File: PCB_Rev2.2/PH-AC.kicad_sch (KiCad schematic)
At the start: 42 parts, among them J1 USB_C_Receptacle_USB2.0_16P, J2 Conn_01x03, SW1 SW_Push, U1 RP2040, U2 AMS1117-3.3, U3 W25Q16JVSS, Y1 Crystal_GND24

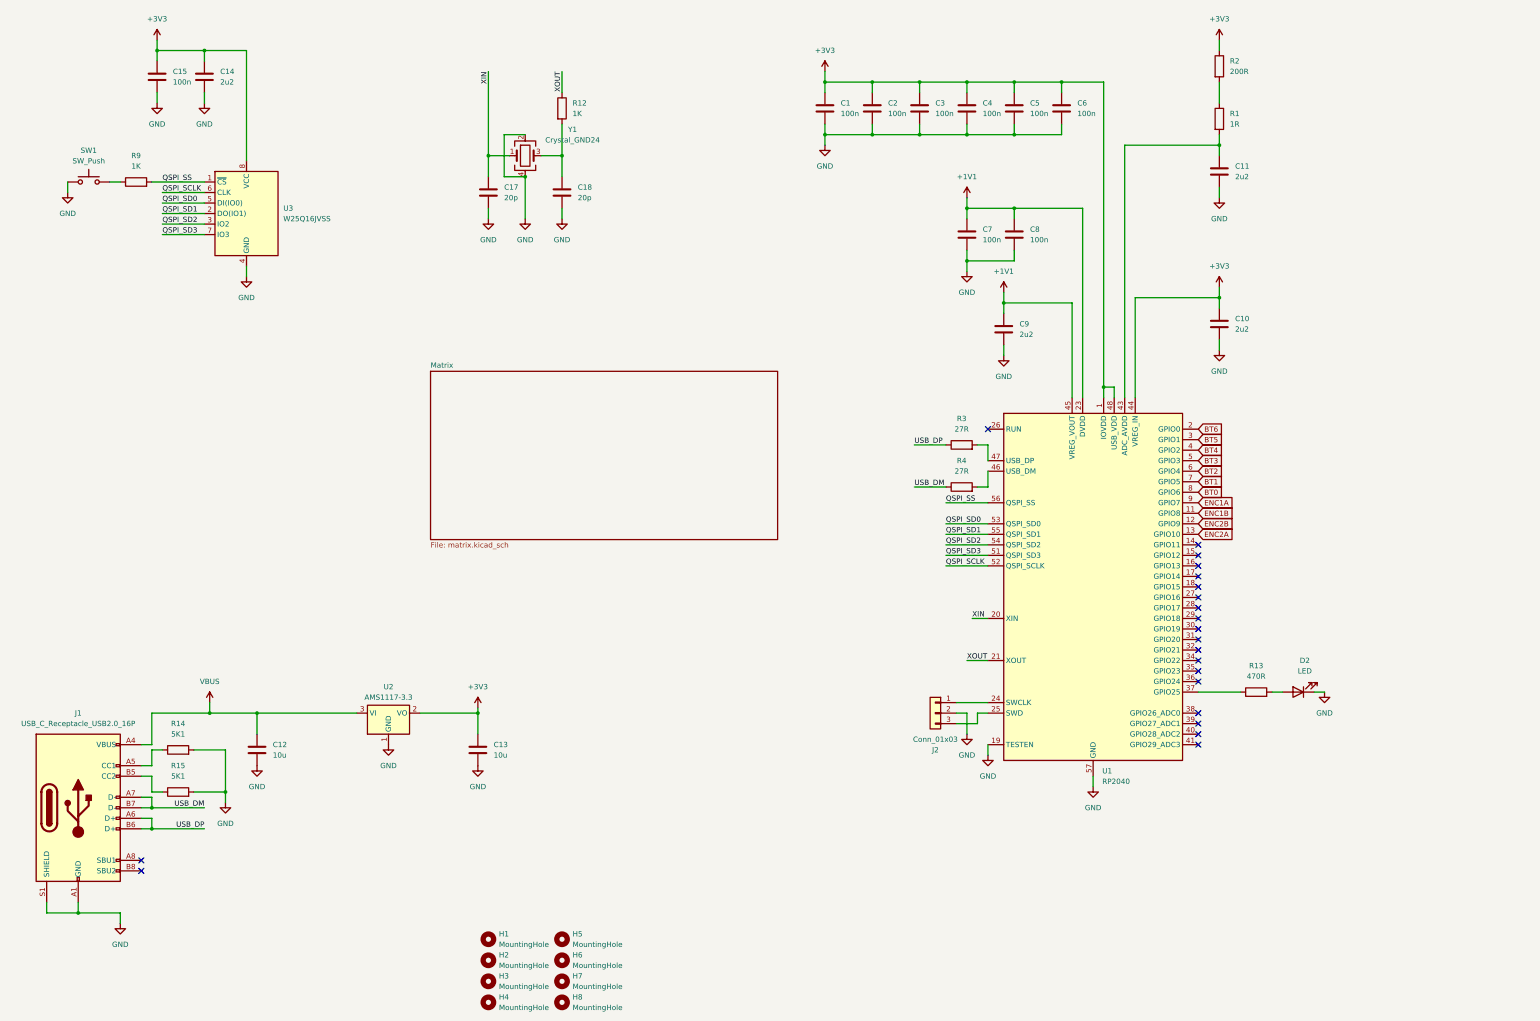
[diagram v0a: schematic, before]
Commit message: Redesign
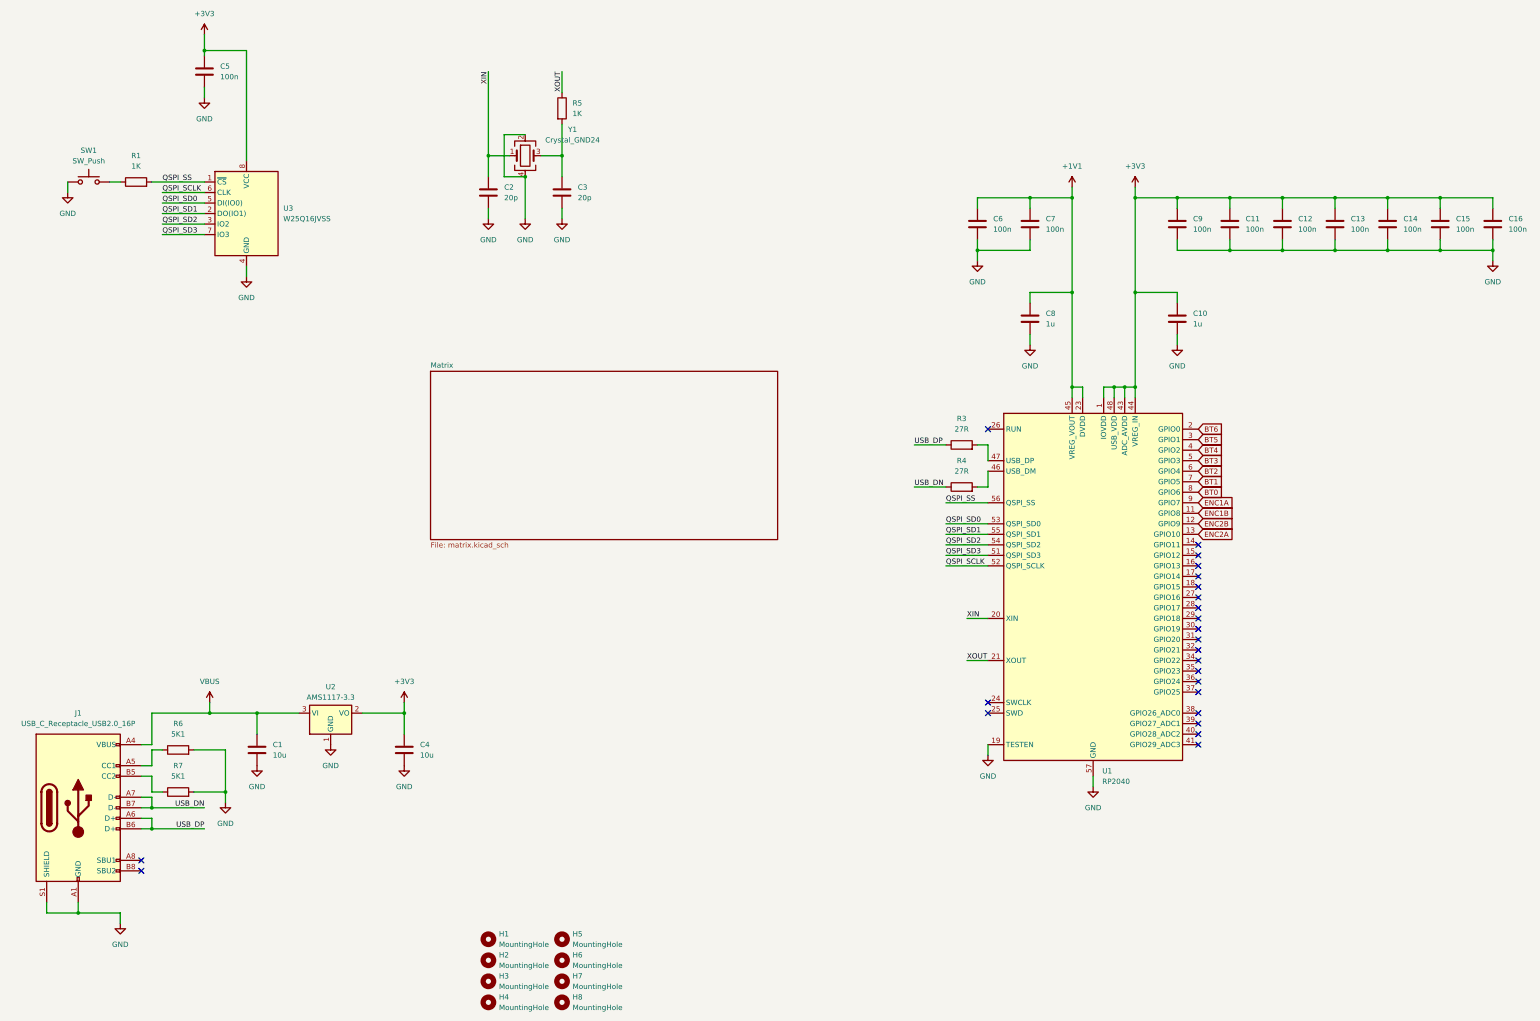
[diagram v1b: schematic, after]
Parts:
- removed C1, C2, C3, C4, C5: 100n, Capacitor_SMD:C_0402_1005Metric, symbol Device:C
- removed D2: LED, LED_SMD:LED_1206_3216Metric, symbol Device:LED
- removed J2: Conn_01x03, Connector_PinHeader_2.54mm:PinHeader_1x03_P2.54mm_Vertical, symbol Connector_Generic:Conn_01x03
- removed R1: 1R, Resistor_SMD:R_0402_1005Metric, symbol Device:R
- removed R13: 470R, Resistor_SMD:R_0402_1005Metric, symbol Device:R
- removed R2: 200R, Resistor_SMD:R_0402_1005Metric, symbol Device:R
- added C12, C13, C15, C16: 100n, Capacitor_SMD:C_0402_1005Metric, symbol Device:C
- C10: value 2u2 -> 1u
- C11, C14, C9: value 2u2 -> 100n
- C8: value 100n -> 1u
- renumbered C12 to C1, C17 to C2, C18 to C3, C13 to C4, C15 to C5, R9 to R1, R12 to R5, R14 to R6, R15 to R7
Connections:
- net +1V1: now also C6.1; no longer C9.1
- net +3V3: now also C11.1, C9.1, U1.43 (ADC_AVDD), C12.1, C13.1, C15.1, C16.1; no longer C6.1
- net GND: now also C12.2, C13.2, C15.2, C16.2
- net USB_DM renamed USB_DN
- no-connect marks 21 -> 24
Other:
- moved on the sheet: C4, C5, U2

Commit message: Revert "Redesign"
This reverts commit 8763a19c73a96b1086359286b52022891444512d.
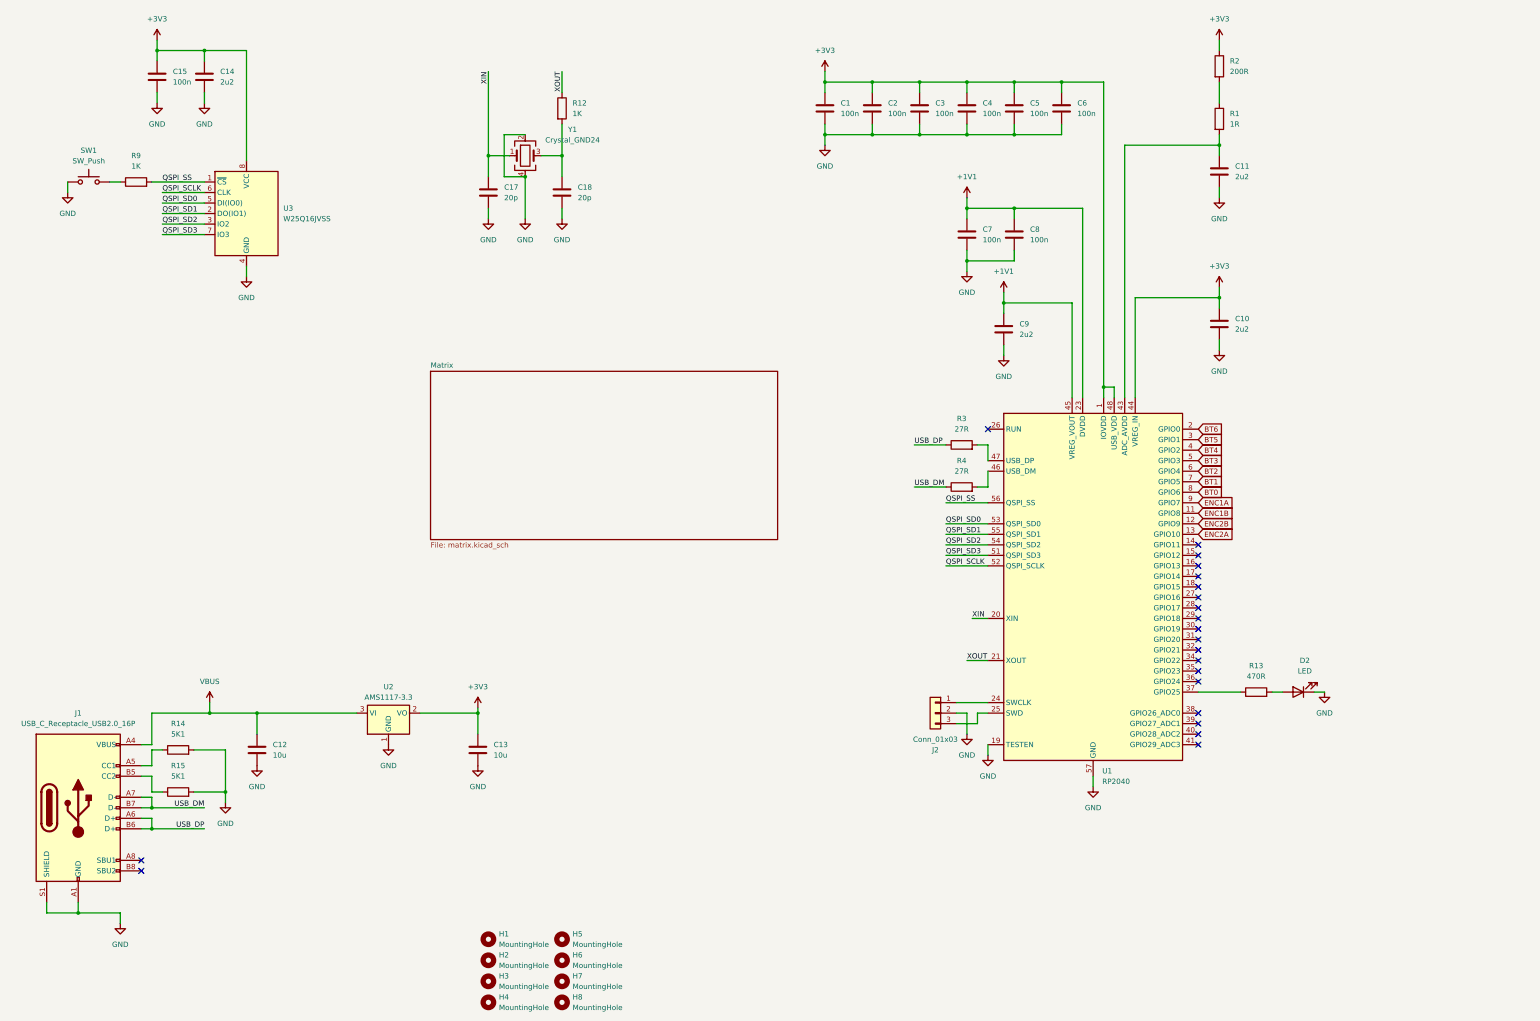
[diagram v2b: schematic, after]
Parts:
- removed C12, C13, C15, C16: 100n, Capacitor_SMD:C_0402_1005Metric, symbol Device:C
- added C1, C2, C3, C4, C5: 100n, Capacitor_SMD:C_0402_1005Metric, symbol Device:C
- added D2: LED, LED_SMD:LED_1206_3216Metric, symbol Device:LED
- added J2: Conn_01x03, Connector_PinHeader_2.54mm:PinHeader_1x03_P2.54mm_Vertical, symbol Connector_Generic:Conn_01x03
- added R1: 1R, Resistor_SMD:R_0402_1005Metric, symbol Device:R
- added R13: 470R, Resistor_SMD:R_0402_1005Metric, symbol Device:R
- added R2: 200R, Resistor_SMD:R_0402_1005Metric, symbol Device:R
- C10: value 1u -> 2u2
- C11, C14, C9: value 100n -> 2u2
- C8: value 1u -> 100n
- renumbered C1 to C12, C4 to C13, C5 to C15, C2 to C17, C3 to C18, R5 to R12, R6 to R14, R7 to R15, R1 to R9
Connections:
- net +1V1: now also C9.1; no longer C6.1
- net +3V3: now also C6.1, C1.1, C2.1, C3.1, C4.1, C5.1, R2.1; no longer C11.1, C9.1, U1.43 (ADC_AVDD)
- net GND: now also C1.2, C2.2, C3.2, C4.2, C5.2, D2.1 (K), J2.2 (Pin_2)
- net at U1.24 (SWCLK): now also J2.1 (Pin_1)
- net at U1.25 (SWD): now also J2.3 (Pin_3)
- net at U1.37 (GPIO25): now also R13.1
- net USB_DN renamed USB_DM
- new net: R1.1, R2.2
- new net: C11.1, R1.2, U1.43 (ADC_AVDD)
- new net: D2.2 (A), R13.2
- no-connect marks 24 -> 21
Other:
- moved on the sheet: C13, C15, U2
